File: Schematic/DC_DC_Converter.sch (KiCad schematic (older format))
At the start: 38 parts, among them Q1 DMG3402L, Q2 DMG3402L, Q3 DMG3402L, Q4 DMG3402L

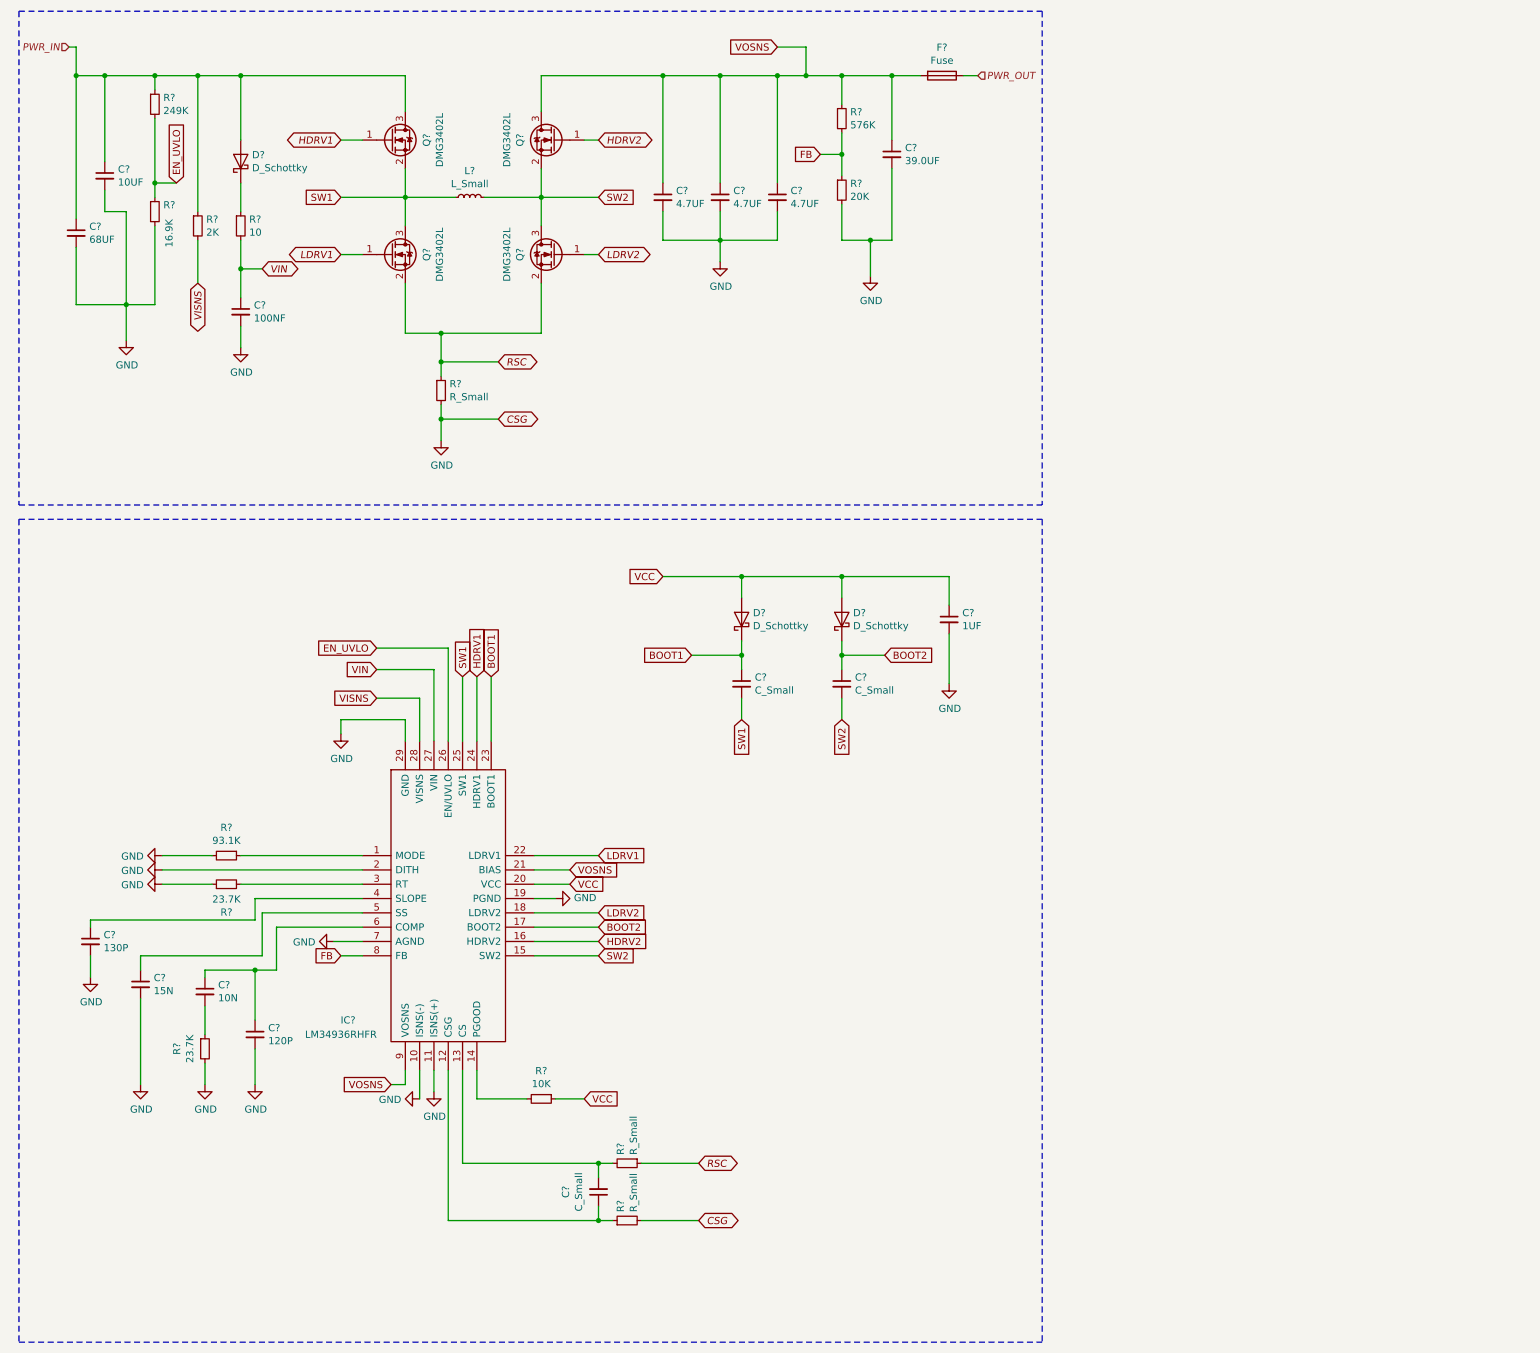
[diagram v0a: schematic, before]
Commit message: Add files via upload
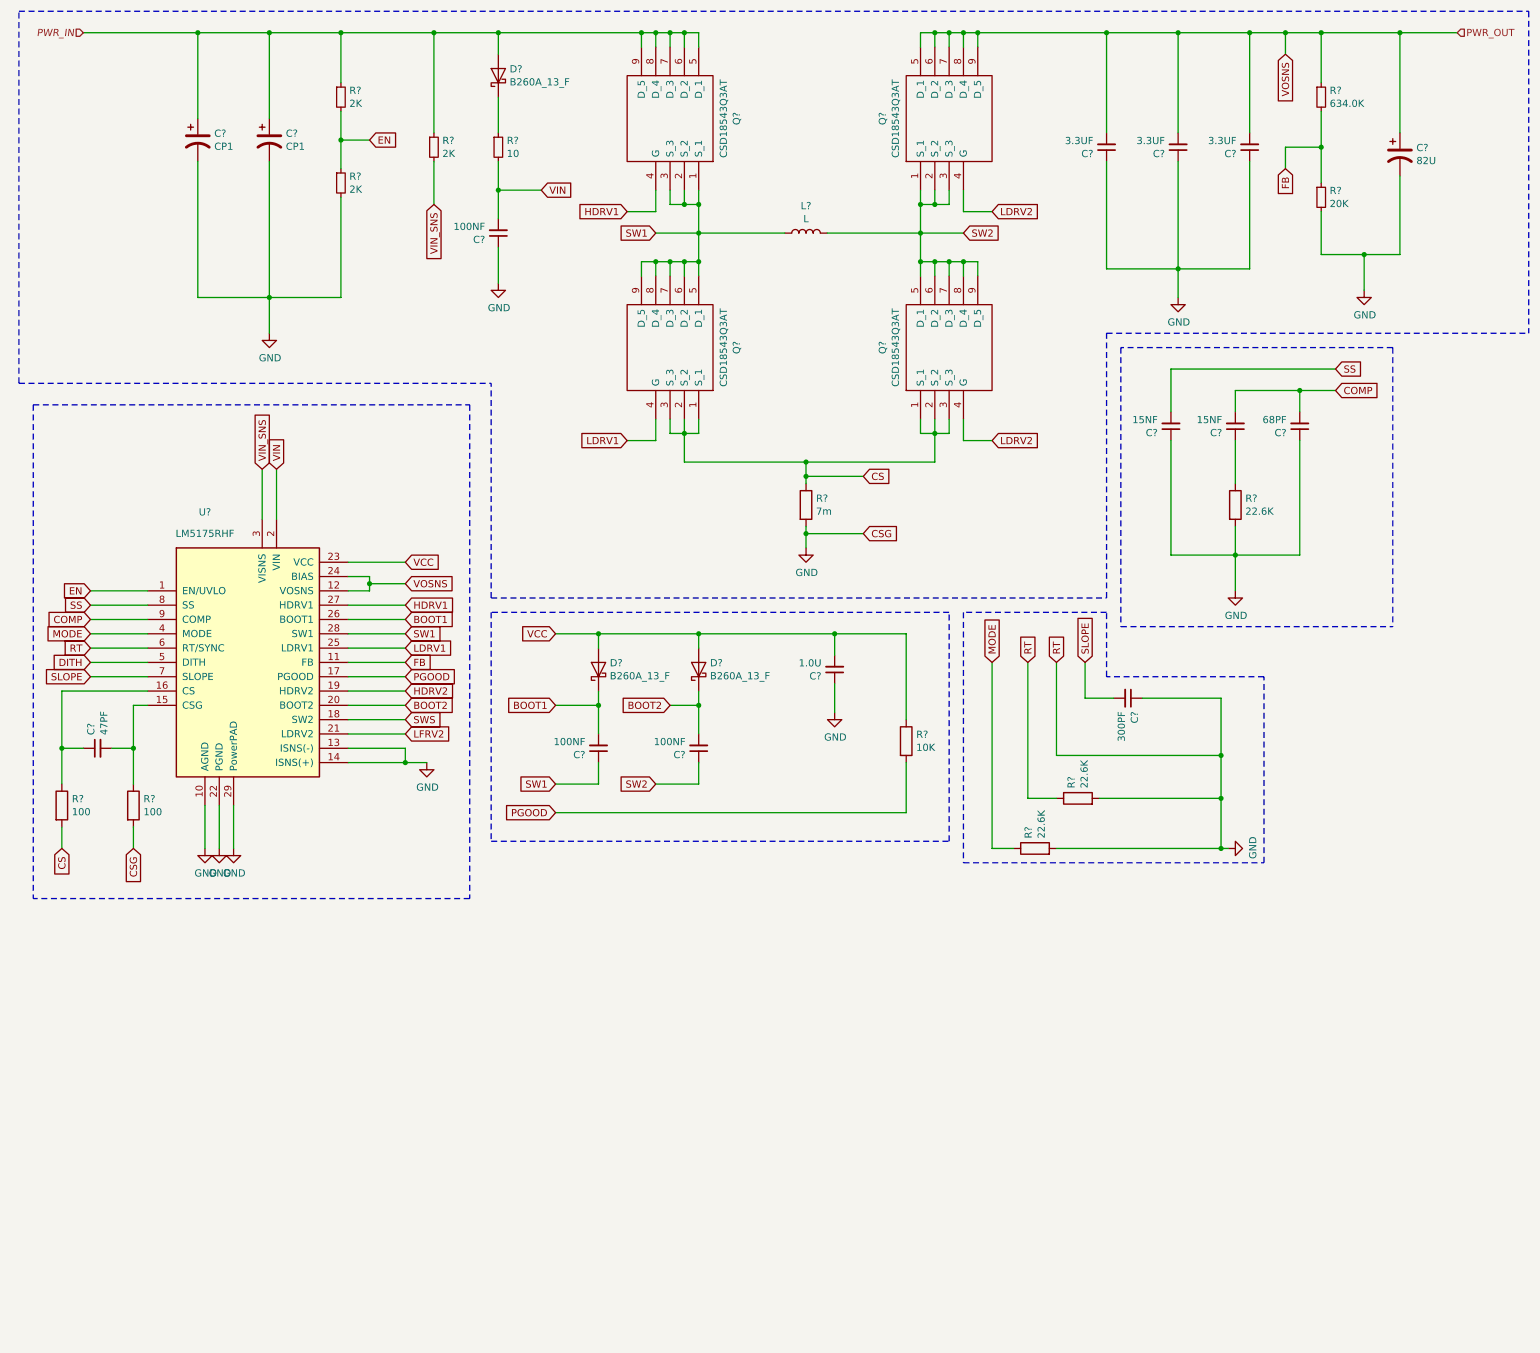
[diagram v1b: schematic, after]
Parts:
- removed C? (x3): C_Small, symbol Device:C_Small
- removed C? (x3): 4.7UF, symbol Device:C_Small
- removed C?: 39.0UF, symbol Device:C_Small
- removed C?: 100NF, symbol Device:C_Small
- removed C?: 10UF, symbol Device:C_Small
- removed C?: 68UF, symbol Device:C_Small
- removed C?: 130P, symbol Device:C_Small
- removed C?: 15N, symbol Device:C_Small
- removed C?: 10N, symbol Device:C_Small
- removed C?: 120P, symbol Device:C_Small
- removed C?: 1UF, symbol Device:C_Small
- removed D? (x3): D_Schottky, symbol Device:D_Schottky
- removed F?: Fuse, symbol Device:Fuse
- removed IC?: LM34936RHFR, ASSETS:QFN50P400X500X100-29N-D, symbol Regular_Use:LM34936RHFR
- removed L?: L_Small, symbol Device:L_Small
- removed Q1, Q2, Q3, Q4: DMG3402L, Package_TO_SOT_SMD:SOT-23, symbol Transistor_FET:DMG3402L
- removed R? (x3): R_Small, symbol Device:R_Small
- removed R?: 576K, symbol Device:R_Small
- removed R?: 20K, symbol Device:R_Small
- removed R?: 10, symbol Device:R_Small
- removed R?: 2K, symbol Device:R_Small
- removed R?: 249K, symbol Device:R_Small
- removed R?: 16.9K, symbol Device:R_Small
- removed R?: 93.1K, symbol Device:R_Small
- removed R? (x2): 23.7K, symbol Device:R_Small
- removed R?: 10K, symbol Device:R_Small
- added C? (x3): 100NF, symbol Device:C_Small
- added C? (x2): CP1, symbol Device:CP1
- added C? (x3): 3.3UF, symbol Device:C_Small
- added C?: 82U, symbol Device:CP1
- added C?: 1.0U, symbol Device:C_Small
- added C?: 47PF, symbol Device:C_Small
- added C? (x2): 15NF, symbol Device:C_Small
- added C?: 68PF, symbol Device:C_Small
- added C?: 300PF, symbol Device:C_Small
- added D? (x3): B260A_13_F, symbol Device:D_Schottky
- added L?: L, symbol Device:L
- added Q? (x4): CSD18543Q3AT, ASSETS:CSD18543Q3AT, symbol Regular_Use:CSD18543Q3AT
- added R?: 7m, symbol Device:R
- added R?: 10, symbol Device:R_Small
- added R? (x3): 2K, symbol Device:R_Small
- added R?: 634.0K, symbol Device:R_Small
- added R?: 20K, symbol Device:R_Small
- added R?: 10K, symbol Device:R
- added R? (x2): 100, symbol Device:R
- added R? (x3): 22.6K, symbol Device:R
- added U?: LM5175RHF, Package_DFN_QFN:VQFN-28-1EP_4x5mm_P0.5mm_EP2.55x3.55mm, symbol Regulator_Switching:LM5175RHF
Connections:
- net BOOT1: now also C?.2, D?.1 (K), U?.26 (BOOT1)
- net BOOT2: now also C?.2, D?.1 (K), U?.20 (BOOT2)
- net FB: now also R?.1, R?.2, U?.11 (FB)
- net GND: now also C?.1, C?.1, C?.1, C?.1, C?.1, C?.1, C?.1, C?.1, C?.2, C?.2, C?.2, R?.1, R?.2, R?.2, R?.2, R?.2, R?.2, R?.2, R?.2, U?.10 (AGND), U?.13 (ISNS(-)), U?.14 (ISNS(+)), U?.22 (PGND), U?.29 (PowerPAD), U?.6 (RT/SYNC)
- net HDRV1: now also Q?.4 (G), U?.27 (HDRV1)
- net HDRV2: now also U?.19 (HDRV2)
- net LDRV1: now also Q?.4 (G), U?.25 (LDRV1)
- net LDRV2: now also Q?.4 (G), Q?.4 (G)
- net PWR_IN: now also C?.1, C?.1, D?.2 (A), Q?.5 (D_1), Q?.6 (D_2), Q?.7 (D_3), Q?.8 (D_4), Q?.9 (D_5), R?.1, R?.1
- net SW1: now also C?.1, L?.1, Q?.1 (S_1), Q?.2 (S_2), Q?.3 (S_3), Q?.5 (D_1), Q?.6 (D_2), Q?.7 (D_3), Q?.8 (D_4), Q?.9 (D_5), U?.28 (SW1)
- net SW2: now also C?.1, L?.2, Q?.1 (S_1), Q?.2 (S_2), Q?.3 (S_3), Q?.5 (D_1), Q?.6 (D_2), Q?.7 (D_3), Q?.8 (D_4), Q?.9 (D_5)
- net VCC: now also C?.2, D?.2 (A), D?.2 (A), R?.1, U?.23 (VCC)
- net VIN: now also C?.2, R?.2, U?.2 (VIN)
- net VOSNS: now also C?.1, C?.2, C?.2, C?.2, Q?.5 (D_1), Q?.6 (D_2), Q?.7 (D_3), Q?.8 (D_4), Q?.9 (D_5), R?.1, U?.12 (VOSNS), U?.24 (BIAS)
- new net: C?.2, R?.1, U?.15 (CSG)
- new net: C?.1, R?.1, U?.16 (CS)
- new net: D?.1 (K), R?.1
- new net: C?.1, R?.1
- new net COMP: C?.2, C?.2, U?.9 (COMP)
- new net CS: Q?.1 (S_1), Q?.1 (S_1), Q?.2 (S_2), Q?.2 (S_2), Q?.3 (S_3), Q?.3 (S_3), R?.1, R?.2
- new net DITH: U?.5 (DITH)
- new net EN: R?.1, R?.2, U?.1 (EN/UVLO)
- new net LFRV2: U?.21 (LDRV2)
- new net MODE: R?.1, U?.4 (MODE)
- new net PGOOD: R?.2, U?.17 (PGOOD)
- new net SLOPE: C?.2, U?.7 (SLOPE)
- new net SS: C?.2, U?.8 (SS)
- new net SWS: U?.18 (SW2)
- new net VIN_SNS: R?.2, U?.3 (VISNS)
